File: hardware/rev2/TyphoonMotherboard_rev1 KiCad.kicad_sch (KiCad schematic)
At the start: 76 parts, among them J1 Conn_02x04_Odd_Even, J2 Conn_01x04_Pin, J3 UJ20-C-H-C-4-SMT-TR, J5 Conn_01x02_Pin, J6 Conn_01x02_Pin, J7 Conn_01x04_Pin, SW1 SW_Push, SW2 SW_Push, SW3 SW_Push, U1 USBLC6-2SC6, U2 ESP32-S3-WROOM-1, U3 SN65HVD233, U4 BQ25798RQMR, U5 TPS62130, U6 TPS62130

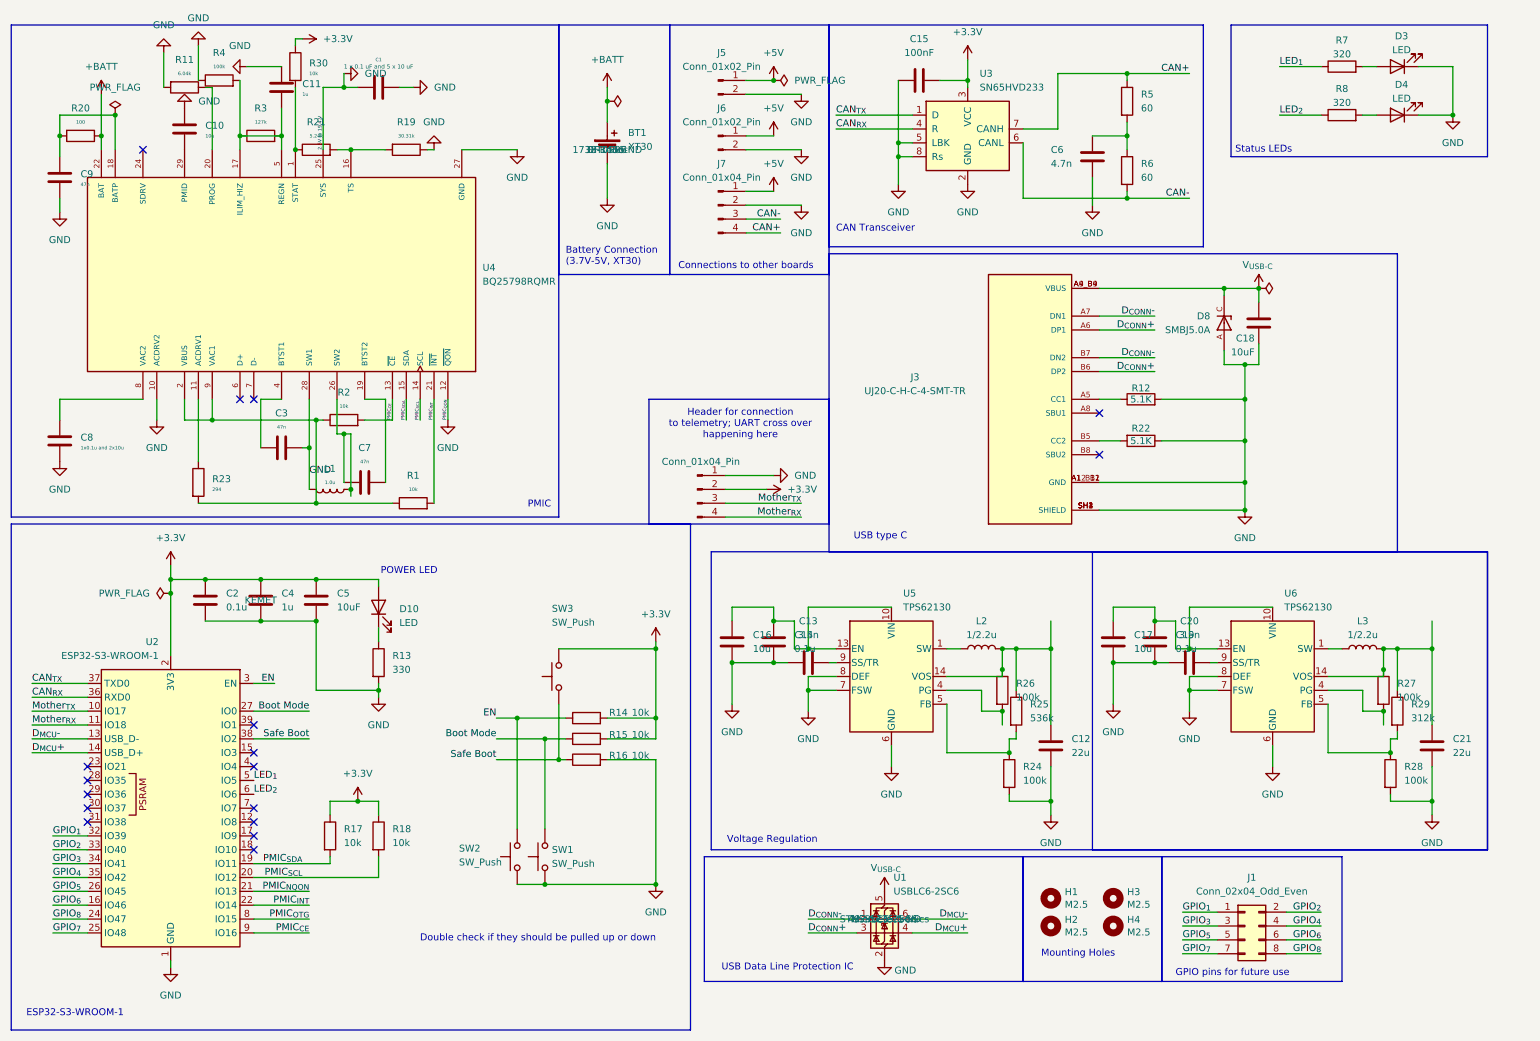
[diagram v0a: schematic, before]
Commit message: removed updates
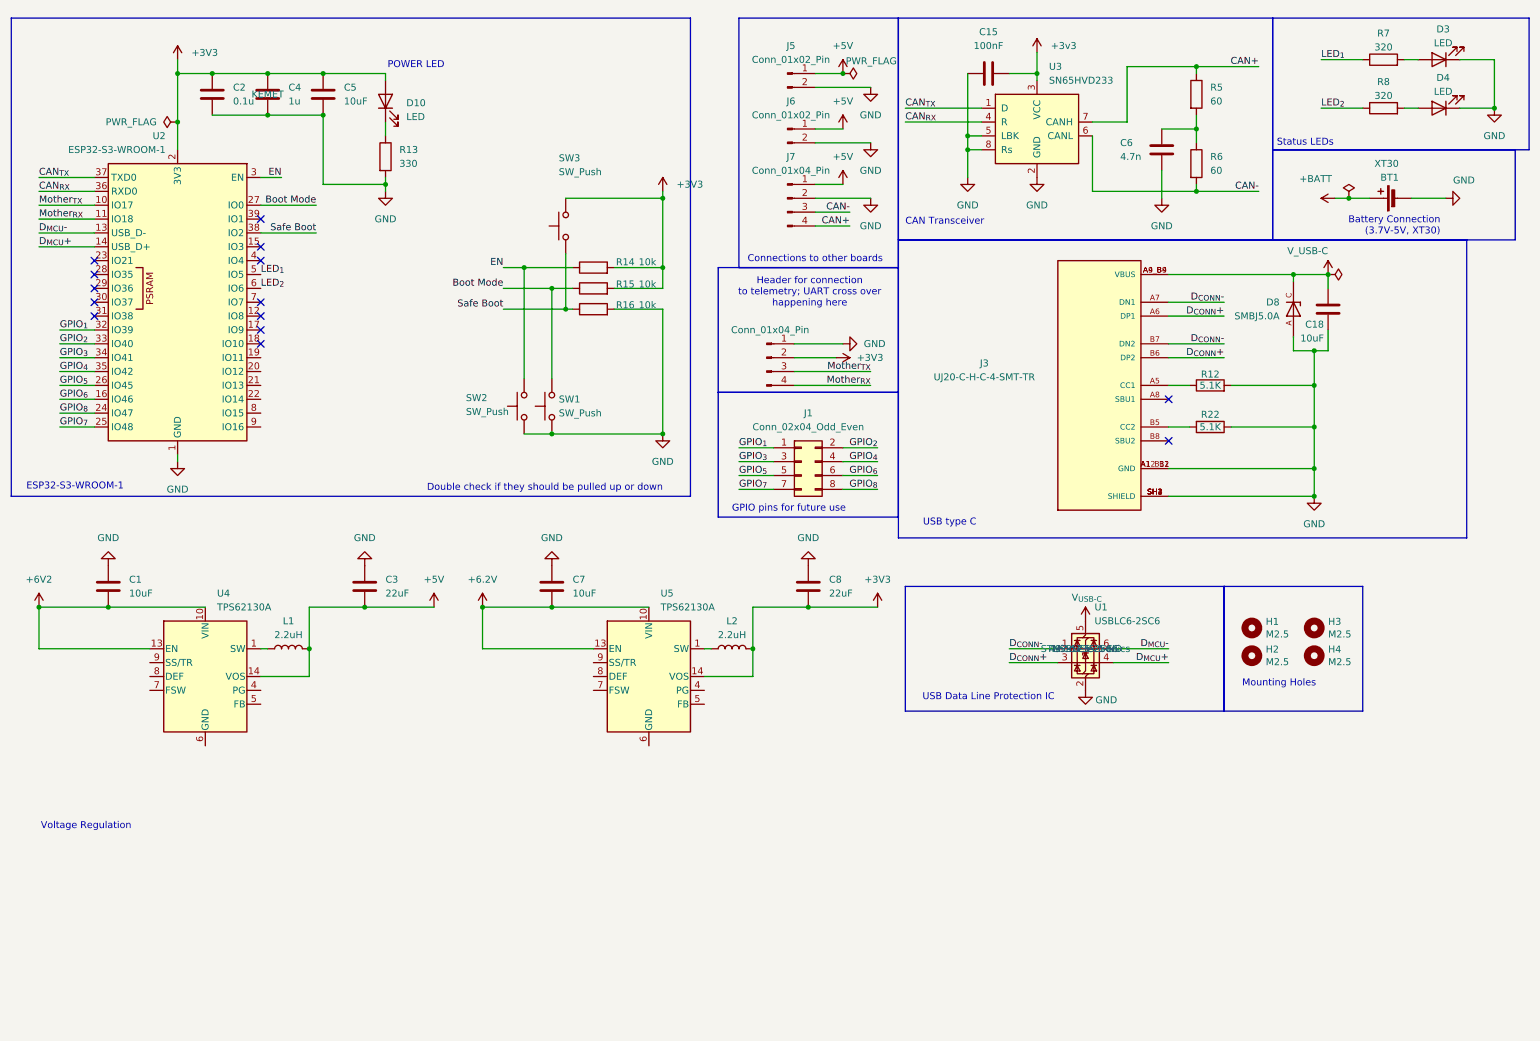
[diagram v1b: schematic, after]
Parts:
- removed C10, C16, C17: 10u, symbol Device:C
- removed C11: 1u, symbol Device:C
- removed C12, C21: 22u, symbol Device:C
- removed C13, C20: 3.5n, symbol Device:C
- removed C14, C19: 0.1u, symbol Device:C
- removed C9: 47n, symbol Device:C
- removed L3: 1/2.2u, symbol Device:L
- removed R1, R2, R30: 10k, symbol Device:R
- removed R11: 6.04k, symbol Device:R
- removed R17, R18: 10k, Resistor_SMD:R_0603_1608Metric, symbol Device:R
- removed R19: 30.31k, symbol Device:R
- removed R20: 100, symbol Device:R
- removed R21: 5.24k, symbol Device:R
- removed R23: 294, symbol Device:R
- removed R24, R26, R27, R28, R4: 100k, symbol Device:R
- removed R25: 536k, symbol Device:R
- removed R29: 312k, symbol Device:R
- removed R3: 127k, symbol Device:R
- removed U4: BQ25798RQMR, BQ25798RQMR:IC_BQ25798RQMR, symbol BQ25798RQMR:BQ25798RQMR
- removed U5, U6: TPS62130, Package_DFN_QFN:VQFN-16-1EP_3x3mm_P0.5mm_EP1.68x1.68mm_ThermalVias, symbol Regulator_Switching:TPS62130
- added U4, U5: TPS62130A, Package_DFN_QFN:VQFN-16-1EP_3x3mm_P0.5mm_EP1.68x1.68mm_ThermalVias, symbol Regulator_Switching:TPS62130A
- C1: value 1 x 0.1 uF and 5 x 10 uF -> 10uF
- C3: value 47n -> 22uF
- C7: value 47n -> 10uF
- C8: value 1x0.1u and 2x10u -> 22uF
- L1: value 1.0u -> 2.2uH
- L2: value 1/2.2u -> 2.2uH
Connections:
- net +5V: now also C3.2, L1.2, U4.14 (VOS)
- net GND: now also C3.1, C7.1, C8.1; no longer C1.2, C3.2, C8.2, L1.2
- net V_{USB-C}: no longer C18.1, D8.C, J3.A4_B9 (VBUS), J3.A9_B4 (VBUS)
- net at L2.1: now also U5.1 (SW), U5.2 (SW), U5.3 (SW)
- net +3V3: now reaches L2.2
- net +3V3: now also C2.1, C4.1, C5.1, C8.2, D10.2 (A), J2.2 (Pin_2), R14.2, R15.2, SW3.2, U2.2 (3V3), U5.14 (VOS)
- net +6.2V: now reaches C7.2
- net +6.2V: now also U5.10 (VIN), U5.11 (VIN), U5.12 (VIN), U5.13 (EN)
- net at L1.1: now also U4.1 (SW), U4.2 (SW), U4.3 (SW); no longer C7.1
- removed net +3.3V: C15.2, C2.1, C4.1, C5.1, D10.2 (A), J2.2 (Pin_2), R14.2, R15.2, SW3.2, U2.2 (3V3), U3.3 (VCC)
- net PMIC_{CE}: no longer names the net of U2.9 (IO16)
- net PMIC_{INT}: no longer names the net of U2.22 (IO14)
- net PMIC_{NQON}: no longer names the net of U2.21 (IO13)
- net PMIC_{OTG}: no longer names the net of U2.8 (IO15)
- net PMIC_{SCL}: no longer names the net of U2.20 (IO12)
- net PMIC_{SDA}: no longer names the net of U2.19 (IO11)
- new net: U4.15 (GND), U4.16 (GND), U4.17 (GND), U4.6 (GND)
- new net: U5.15 (GND), U5.16 (GND), U5.17 (GND), U5.6 (GND)
- new net +3v3: C15.2, U3.3 (VCC)
- new net +6V2: C1.2, U4.10 (VIN), U4.11 (VIN), U4.12 (VIN), U4.13 (EN)
- new net V_USB-C: C18.1, D8.C, J3.A4_B9 (VBUS), J3.A9_B4 (VBUS)
- no-connect marks 17 -> 14
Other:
- note removed: "PMIC"
- moved on the sheet: BT1, C15, C18, C2, C4, C5, C6, D10, D3, D4, D8, H1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
